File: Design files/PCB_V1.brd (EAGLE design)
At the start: 92.4 x 94 mm, 48 parts, among them IC2 786TV, T1 BC337, T2 BC337, T3 BC337, T4 BC337, X1 1-227161-0, X2 1-227161-0, X3 1-227161-0, X4 1-227161-0, X5 1-227161-0, X6 1-227161-0, X7 1-227161-0, X8 1-227161-0

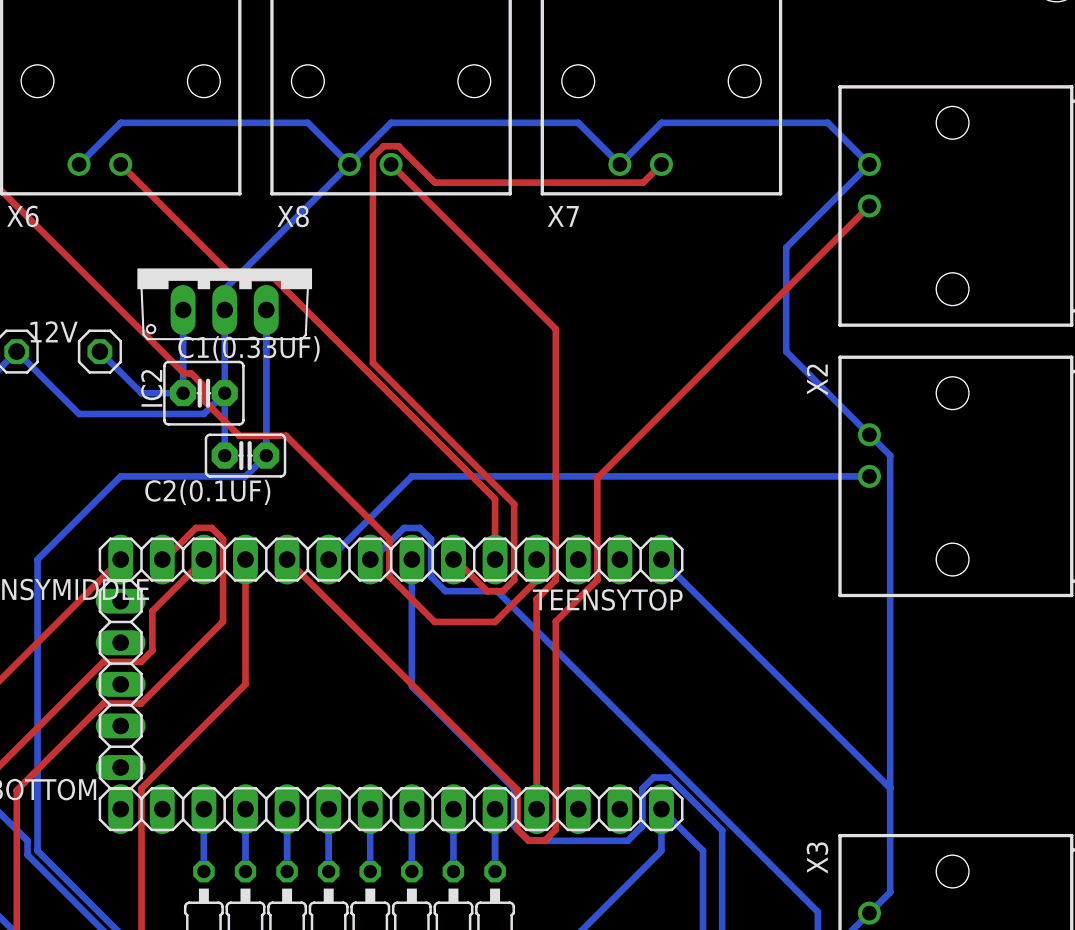
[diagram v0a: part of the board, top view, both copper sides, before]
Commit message: V2
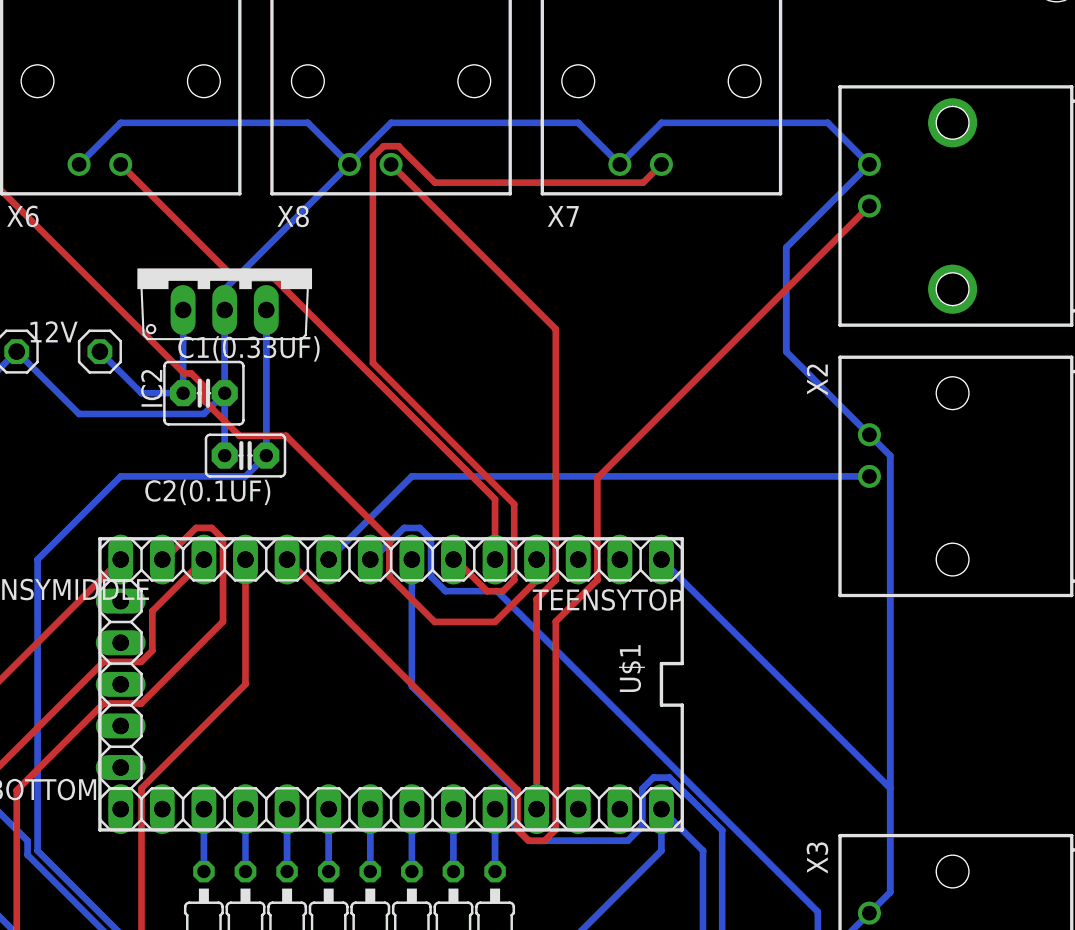
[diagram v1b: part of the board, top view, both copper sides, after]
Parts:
- added U$1: TEENSY_LC_OUTER_ROW, Teensy_3_and_LC_Series_Boards_v1.4:TEENSY_3.0-3.2&LC_OUTER_ROW
- X1: device con-coax:AMP_227161 -> con-coax_xavi:AMP_227161
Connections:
- new net 26/A12/DAC: U$1.RESET/DAC
- new net 3.3V: U$1.3.3V, U$1.3.3V1
- new net GND: U$1.AGND, U$1.GND, U$1.GND1
- new net VIN: U$1.VIN
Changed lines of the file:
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@@
 <attribute name="VALUE" x="4.445" y="48.26" size="1.27" layer="27" rot="R270"/>
 </element>
-<element name="X1" library="con-coax" library_urn="urn:adsk.eagle:library:133" package="AMP_227161" package3d_urn="urn:adsk.eagle:package:6212/1" value="1-227161-0" x="58.42" y="71.12" smashed="yes" rot="R270">
+<element name="X1" library="con-coax_xavi" package="AMP_227161" package3d_urn="urn:adsk.eagle:package:6212/1" value="1-227161-0" x="58.42" y="71.12" smashed="yes" rot="R270">
 <attribute name="MF" value="TYCO ELECTRONICS" x="48.26" y="48.26" size="1.778" layer="27" rot="R270" display="off"/>
 <attribute name="MPN" value="1-227161" x="48.26" y="48.26" size="1.778" layer="27" rot="R270" display="off"/>
@@
 <attribute name="POPULARITY" value="0" x="-54.61" y="156.21" size="1.778" layer="27" display="off"/>
 <attribute name="VALUE" x="23.495" y="69.85" size="1.27" layer="27"/>
+</element>
+<element name="U$1" library="Teensy_3_and_LC_Series_Boards_v1.4" package="TEENSY_3.0-3.2&amp;LC_OUTER_ROW" value="TEENSY_LC_OUTER_ROW" x="24.13" y="41.91" smashed="yes" rot="R270">
+<attribute name="NAME" x="38.1" y="44.45" size="1.27" layer="25" font="vector" rot="R270"/>
+<attribute name="VALUE" x="10.16" y="45.72" size="1.27" layer="27" font="vector" rot="R270"/>
 </element>
 </elements>
@@
 </polygon>
 </signal>
+<signal name="GND">
+<contactref element="U$1" pad="AGND"/>
+<contactref element="U$1" pad="GND"/>
+<contactref element="U$1" pad="GND1"/>
+<wire x1="38.1" y1="34.29" x2="40.64" y2="49.53" width="0" layer="19" extent="1-1"/>
+<wire x1="7.62" y1="41.91" x2="38.1" y2="34.29" width="0" layer="19" extent="1-1"/>
+</signal>
+<signal name="3.3V">
+<contactref element="U$1" pad="3.3V1"/>
+<contactref element="U$1" pad="3.3V"/>
+<wire x1="7.62" y1="44.45" x2="35.56" y2="34.29" width="0" layer="19" extent="1-1"/>
+</signal>
+<signal name="26/A12/DAC">
+<contactref element="U$1" pad="RESET/DAC"/>
+</signal>
+<signal name="VIN">
+<contactref element="U$1" pad="VIN"/>
+</signal>
 </signals>
